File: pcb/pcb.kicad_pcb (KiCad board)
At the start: 2 copper layers, 76.8 x 75 mm, 38 parts, among them J1 Conn_01x04, SW1 SW_Push, SW10 SW_Push, SW11 SW_Push, SW12 SW_Push, SW2 SW_Push, SW3 SW_Push, SW4 SW_Push, SW5 SW_Push, SW6 SW_Push, SW7 SW_Push, SW8 SW_Push, SW9 SW_Push, U1 XIAO-RP2040-DIP

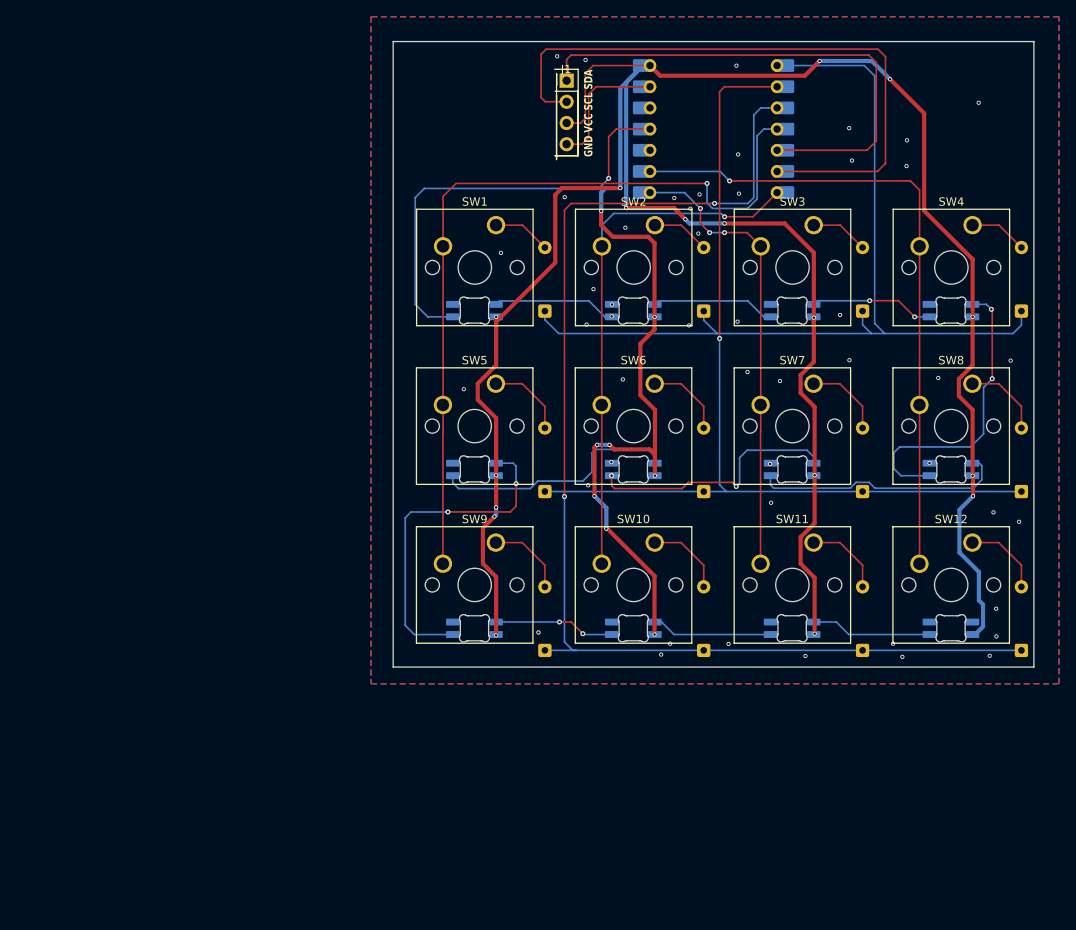
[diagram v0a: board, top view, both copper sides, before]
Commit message: Updated the PCB files
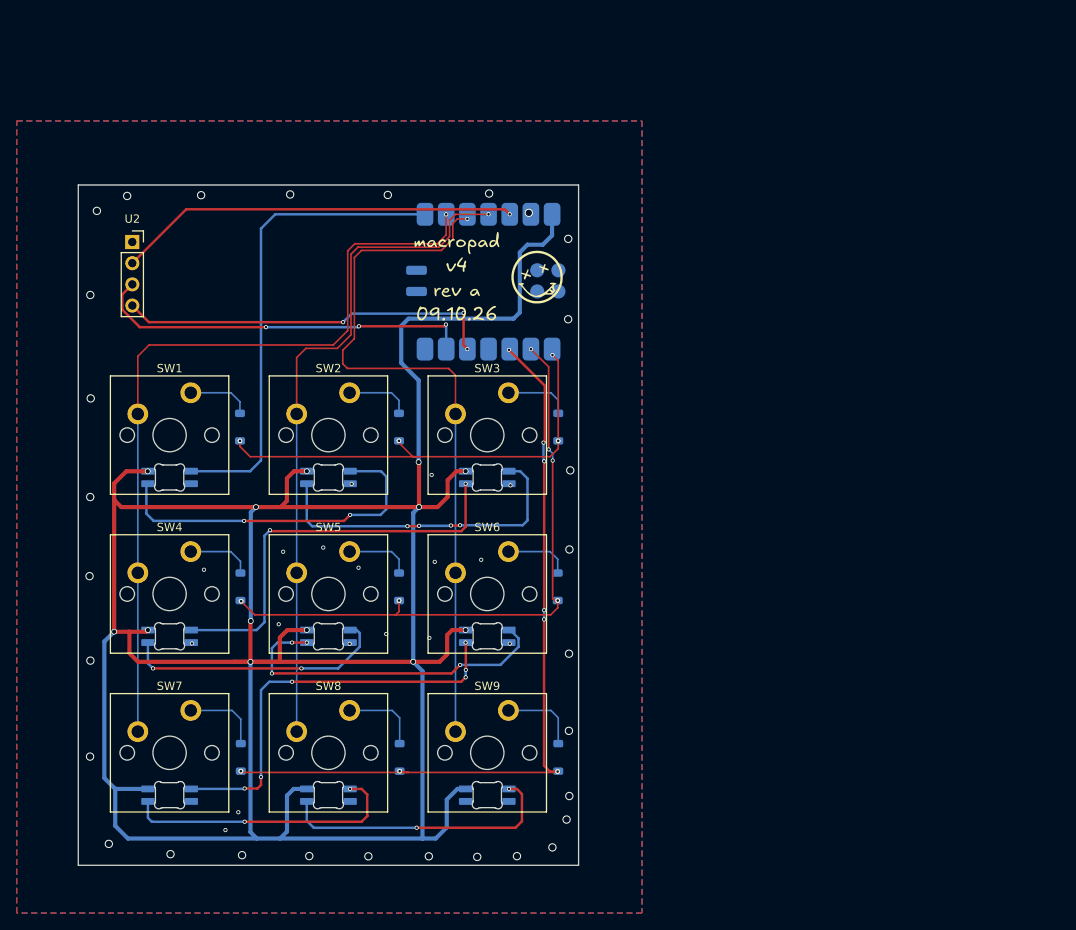
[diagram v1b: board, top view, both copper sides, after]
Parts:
- removed D19, D20, D21, D22, D23, D24: SK6812, KEYS:MX_SK6812MINI-E
- removed J1: Conn_01x04, Connector_PinHeader_2.54mm:PinHeader_1x04_P2.54mm_Vertical
- removed SW10, SW11, SW12: SW_Push, Button_Switch_Keyboard:SW_Cherry_MX_1.00u_PCB
- added G***: LOGO, LOGO, F.Cu at (166.6, 69.0)
- added G***: LOGO, LOGO, B.Cu at (150.3, 68.4)
- added G***: LOGO, LOGO, B.Cu at (135.3, 68.7)
- added U2: OLED_0.91_I2C, Connector_PinSocket_2.54mm:PinSocket_1x04_P2.54mm_Vertical, F.Cu at (123.9, 64.5)
- D1, D2, D3, D4, D5, D6, D7, D8, D9: footprint Diode_THT:D_DO-35_SOD27_P7.62mm_Horizontal -> Diode_SMD:D_SOD-123
- D10, D11, D12: value D -> SK6812MINI-E; footprint Diode_THT:D_DO-35_SOD27_P7.62mm_Horizontal -> SK6812 MINI-E:MX_SK6812MINI-E; moved to F.Cu
- D13, D14, D15, D16, D17, D18: value SK6812 -> SK6812MINI-E; footprint KEYS:MX_SK6812MINI-E -> SK6812 MINI-E:MX_SK6812MINI-E
- SW1, SW2, SW3, SW4, SW5, SW6, SW7, SW8, SW9: value SW_Push -> SW_Push_45deg; footprint Button_Switch_Keyboard:SW_Cherry_MX_1.00u_PCB -> KEYS:SW_Cherry_MX_PCB
- U1: footprint XIAO:XIAO-RP2040-DIP -> XIAO:XIAO-RP2040-SMD
- moved D16 110.3 mm to (128.3, 125.8)
- moved SW4 106.0 mm to (128.3, 106.7)
- moved D4 99.3 mm to (136.8, 105.9)
- moved SW8 89.0 mm to (147.4, 125.8)
- moved SW7 89.0 mm to (128.3, 125.8)
- moved D17 84.3 mm to (147.4, 125.8)
- moved D7 81.1 mm to (136.9, 126.3)
- moved D8 81.1 mm to (155.9, 126.3)
- moved D10 69.1 mm to (128.3, 87.7), turned to 0 degrees
- moved D11 69.1 mm to (147.4, 87.7), turned to 0 degrees
- moved D12 69.1 mm to (166.4, 87.7), turned to 0 degrees
- moved D13 53.5 mm to (128.3, 106.7)
- moved D14 53.5 mm to (147.4, 106.7)
- moved D15 53.5 mm to (166.4, 106.7)
- moved D18 53.5 mm to (166.4, 125.8)
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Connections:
- D1 pad 1: R1 -> /R1
- D10 pad 1: R3 -> GND
- D10 pad 2: Net-(D10-A) -> /DIN
- D11 pad 1: R3 -> GND
- D11 pad 2: Net-(D11-A) -> Net-(D10-DOUT)
- D12 pad 1: R3 -> GND
- D12 pad 2: Net-(D12-A) -> Net-(D11-DOUT)
- D13 pad 2: LED_IN -> Net-(D12-DOUT)
- D18 pad 4: Net-(D18-DOUT) -> unconnected-(D18-DOUT-Pad4)
- D2 pad 1: R1 -> /R1
- D3 pad 1: R1 -> /R1
- D4 pad 1: R1 -> /R2
- D5 pad 1: R2 -> /R2
- D6 pad 1: R2 -> /R2
- D7 pad 1: R2 -> /R3
- D8 pad 1: R2 -> /R3
- D9 pad 1: R3 -> /R3
- SW1 pad 1: Net-(D1-A) -> /C1
- SW1 pad 2: C1 -> Net-(D1-A)
- SW2 pad 1: Net-(D2-A) -> /C2
- SW2 pad 2: C2 -> Net-(D2-A)
- SW3 pad 1: Net-(D3-A) -> /C3
- SW3 pad 2: C3 -> Net-(D3-A)
- SW4 pad 1: Net-(D4-A) -> /C1
- SW4 pad 2: C4 -> Net-(D4-A)
- SW5 pad 1: Net-(D5-A) -> /C2
- SW5 pad 2: C1 -> Net-(D5-A)
- SW6 pad 1: Net-(D6-A) -> /C3
- SW6 pad 2: C2 -> Net-(D6-A)
- SW7 pad 1: Net-(D7-A) -> /C1
- SW7 pad 2: C3 -> Net-(D7-A)
- SW8 pad 1: Net-(D8-A) -> /C2
- SW8 pad 2: C4 -> Net-(D8-A)
- SW9 pad 1: Net-(D9-A) -> /C3
- SW9 pad 2: C1 -> Net-(D9-A)
- U1 pad 1: R1 -> /R1
- U1 pad 10: unconnected-(U1-GPIO4/MISO-Pad10)_1 -> /C3
- U1 pad 11: LED_IN -> /C2
- U1 pad 2: R2 -> /R2
- U1 pad 3: R3 -> /R3
- U1 pad 4: C1 -> unconnected-(U1-GPIO29/ADC3/A3-Pad4)
- U1 pad 5: SDA -> /SDA
- U1 pad 6: SCL -> /SCL
- U1 pad 7: C2 -> unconnected-(U1-GPIO0/TX-Pad7)
- U1 pad 8: C3 -> /DIN
- U1 pad 9: C4 -> /C1
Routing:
- net R3: track 147.1 -> 0.00 mm, vias 2 -> 0
- net R2: track 112.8 -> 0.00 mm, vias 1 -> 0
- net R1: track 110.2 -> 0.00 mm
- net /C1: track 0.00 -> 96.1 mm, vias 0 -> 1
- net C1: track 95.8 -> 0.00 mm, vias 1 -> 0
- net /R3: track 0.00 -> 93.1 mm, vias 0 -> 8
- net /C3: track 0.00 -> 86.7 mm, vias 0 -> 1
- net /C2: track 0.00 -> 81.8 mm, vias 0 -> 1
- net C4: track 78.1 -> 0.00 mm, vias 1 -> 0
- net SCL: track 76.6 -> 0.00 mm
- net /R2: track 0.00 -> 73.8 mm, vias 0 -> 6
- net C2: track 63.6 -> 0.00 mm, vias 1 -> 0
- net SDA: track 62.0 -> 0.00 mm
- net /DIN: track 0.00 -> 57.1 mm
- net C3: track 55.1 -> 0.00 mm, vias 3 -> 0
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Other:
- board size 76.8 x 75 mm -> 60 x 81.6 mm
- board text added: "*Made on Earth by humans*"
